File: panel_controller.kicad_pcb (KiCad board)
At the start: 2 copper layers, 105.5 x 88.5 mm, 17 parts, among them J1 Screw_Terminal_01x04, J2 SSW-104-01-F-S, J3 Screw_Terminal_01x03, J4 Screw_Terminal_01x02, J5 SSW-108-02-G-D, U1 ESP32-DEVKIT-V1

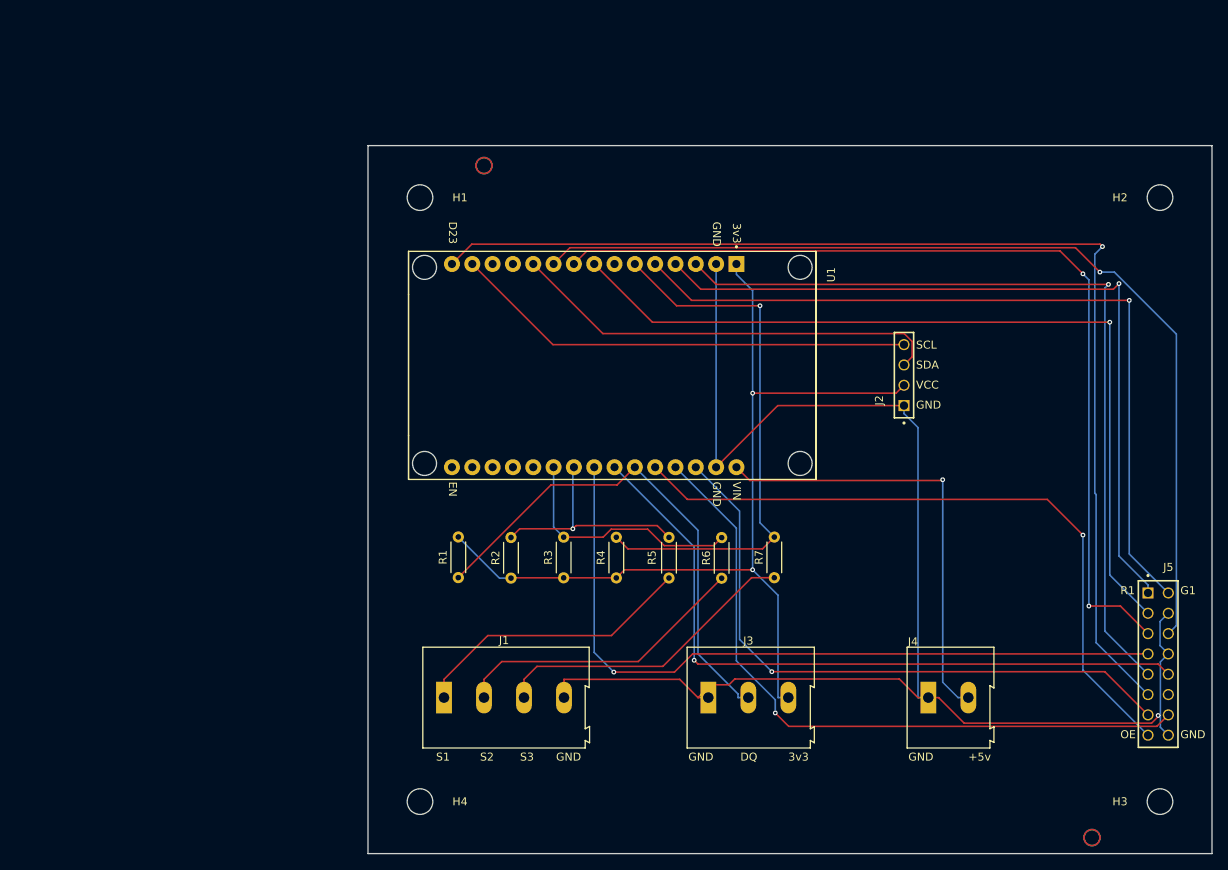
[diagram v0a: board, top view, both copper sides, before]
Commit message: pcb clock v1.5
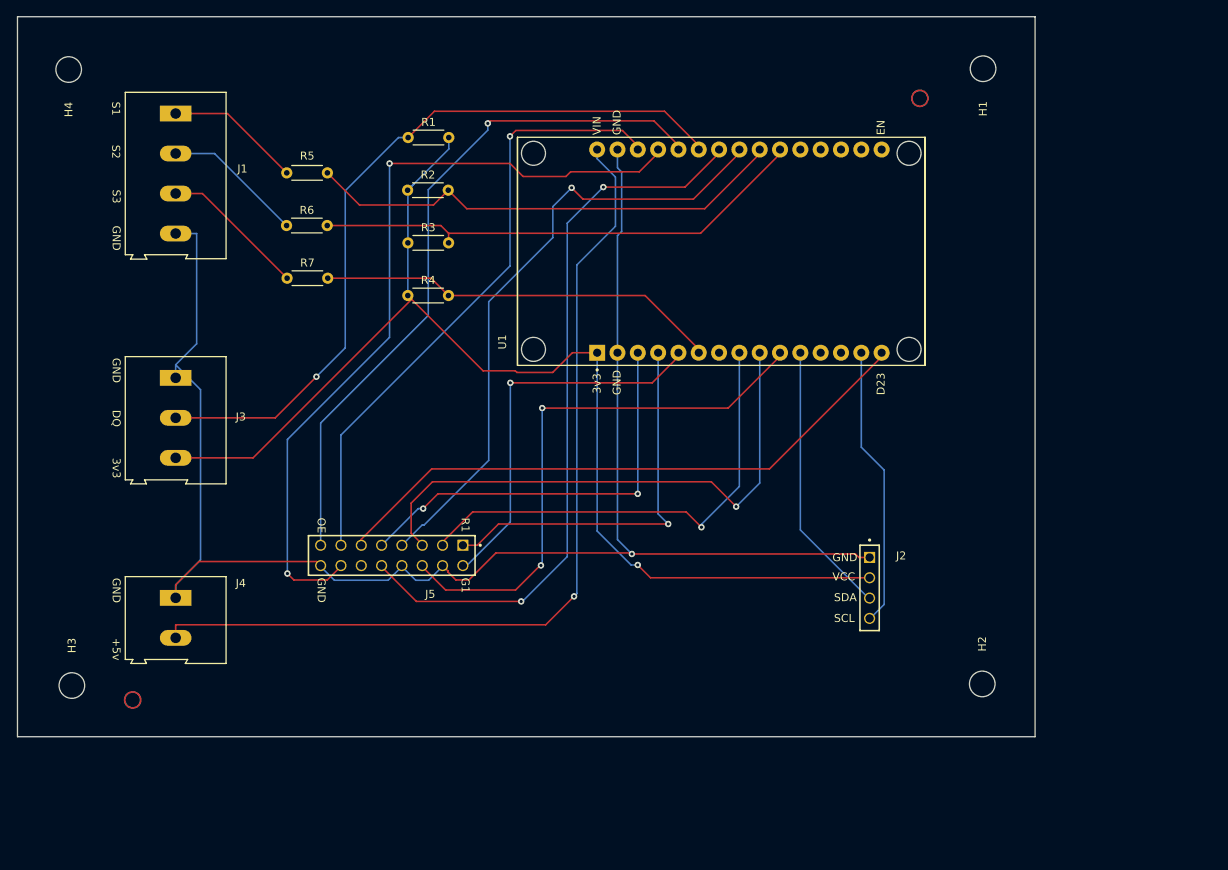
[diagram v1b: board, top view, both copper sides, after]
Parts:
- moved H3 136.8 mm to (82.5, 125.0), turned to 180 degrees
- moved J5 105.8 mm to (121.4, 117.5), turned to -90 degrees
- moved H4 101.5 mm to (82.1, 48.0), turned to 0 degrees
- moved J4 94.9 mm to (95.5, 114.0), turned to -90 degrees
- moved J1 80.3 mm to (95.5, 53.5), turned to -90 degrees
- moved J3 77.7 mm to (95.5, 86.5), turned to -90 degrees
- moved H1 72.2 mm to (196.4, 47.9), turned to 0 degrees
- moved R7 71.5 mm to (109.4, 74.1), turned to 0 degrees
- moved R6 70.0 mm to (109.3, 67.5), turned to 0 degrees
- moved R5 69.6 mm to (109.3, 60.9), turned to 0 degrees
- moved H2 64.7 mm to (196.3, 124.8), turned to 180 degrees
- moved R1 55.4 mm to (124.5, 56.5), turned to 0 degrees
- moved R2 50.2 mm to (124.5, 63.1), turned to 0 degrees
- moved R3 46.2 mm to (124.5, 69.7), turned to 0 degrees
- moved R4 43.9 mm to (124.5, 76.2), turned to 0 degrees
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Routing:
- net Net-(U1-D23): track 141.6 -> 75.7 mm, vias 1 -> 0
- net +5V: track 55.8 -> 111.8 mm
- net Net-(U1-D15): track 103.8 -> 52.3 mm, vias 1 -> 2
- net Net-(U1-D4): track 99.7 -> 48.4 mm
- net Net-(U1-D19): track 121.0 -> 70.0 mm, vias 1 -> 2
- net Net-(U1-D2): track 97.2 -> 48.7 mm
- net Net-(U1-D5): track 105.8 -> 58.9 mm
- net Net-(U1-D18): track 116.1 -> 69.3 mm, vias 2 -> 1
- net Net-(U1-D32): track 30.7 -> 62.9 mm
- net Net-(U1-D33): track 28.7 -> 60.8 mm, vias 1 -> 0
- net Net-(J3-Pin_2): track 63.2 -> 95.0 mm, vias 0 -> 1
- net +3V3: track 116.3 -> 148.1 mm, vias 2 -> 1
- net Net-(U1-D22): track 58.1 -> 35.2 mm
- net Net-(J1-Pin_3): track 38.8 -> 18.3 mm
- net Net-(U1-D21): track 54.7 -> 34.3 mm
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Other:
- board size 105.5 x 88.5 mm -> 127.2 x 90 mm

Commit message: pcb clock v1.6
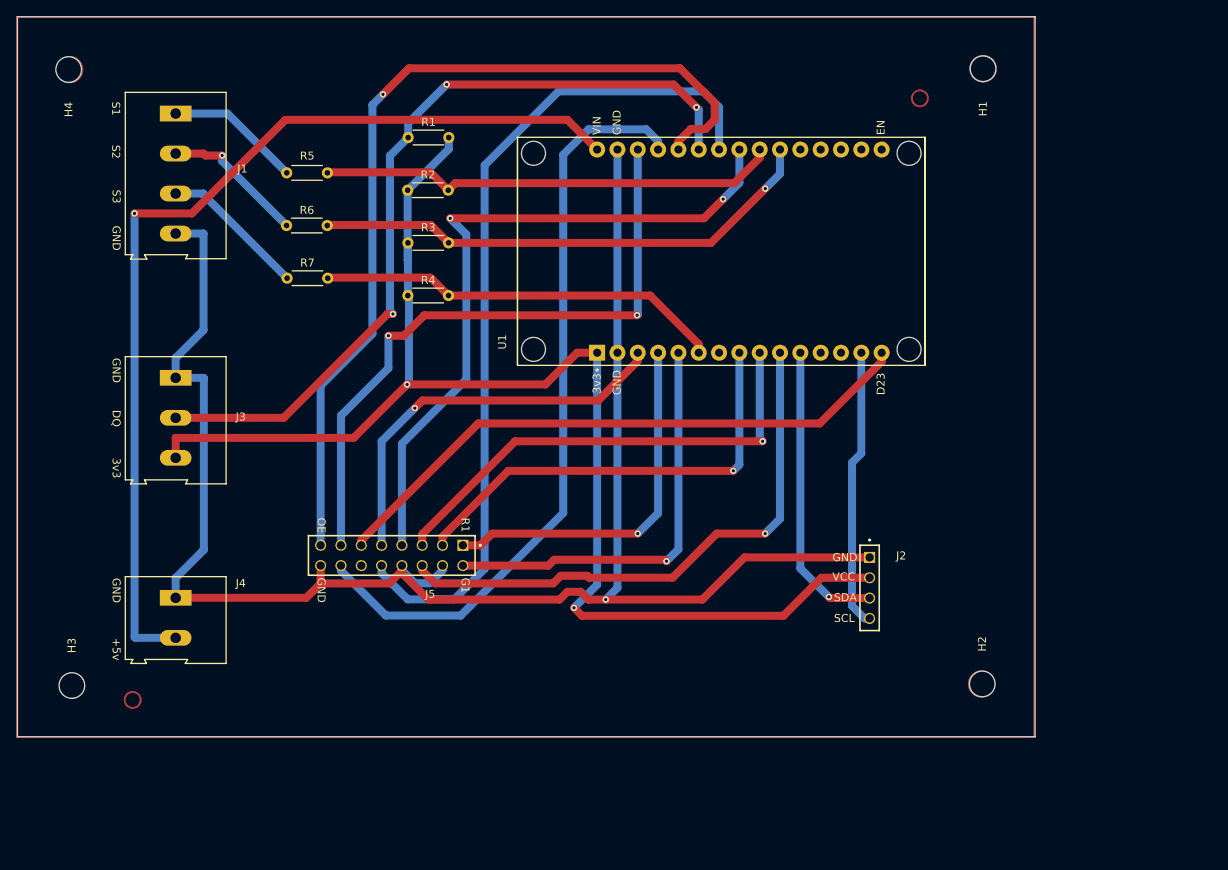
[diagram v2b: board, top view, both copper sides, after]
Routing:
- net Net-(U1-D14): track 87.1 -> 113.0 mm
- net +3V3: track 148.1 -> 167.4 mm, vias 1 -> 2
- net GND: track 200.6 -> 215.5 mm
- net Net-(U1-D26): track 92.2 -> 106.5 mm, vias 2 -> 0
- net +5V: track 111.8 -> 122.3 mm
- net Net-(U1-D18): track 69.3 -> 60.0 mm
- net Net-(U1-D25): track 78.0 -> 87.2 mm, vias 1 -> 2
- net Net-(J3-Pin_2): track 95.0 -> 102.1 mm, vias 1 -> 3
- net Net-(U1-D12): track 100.3 -> 95.7 mm, vias 2 -> 0
- net Net-(U1-D13): track 77.4 -> 81.5 mm, vias 1 -> 2
- net Net-(U1-D4): track 48.4 -> 52.5 mm
- net Net-(U1-D33): track 60.8 -> 57.7 mm
- net Net-(U1-D5): track 58.9 -> 55.9 mm
- net Net-(U1-D21): track 34.3 -> 37.2 mm, vias 0 -> 1
- net Net-(U1-D2): track 48.7 -> 46.1 mm
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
